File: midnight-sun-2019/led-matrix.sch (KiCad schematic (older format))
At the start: 472 parts

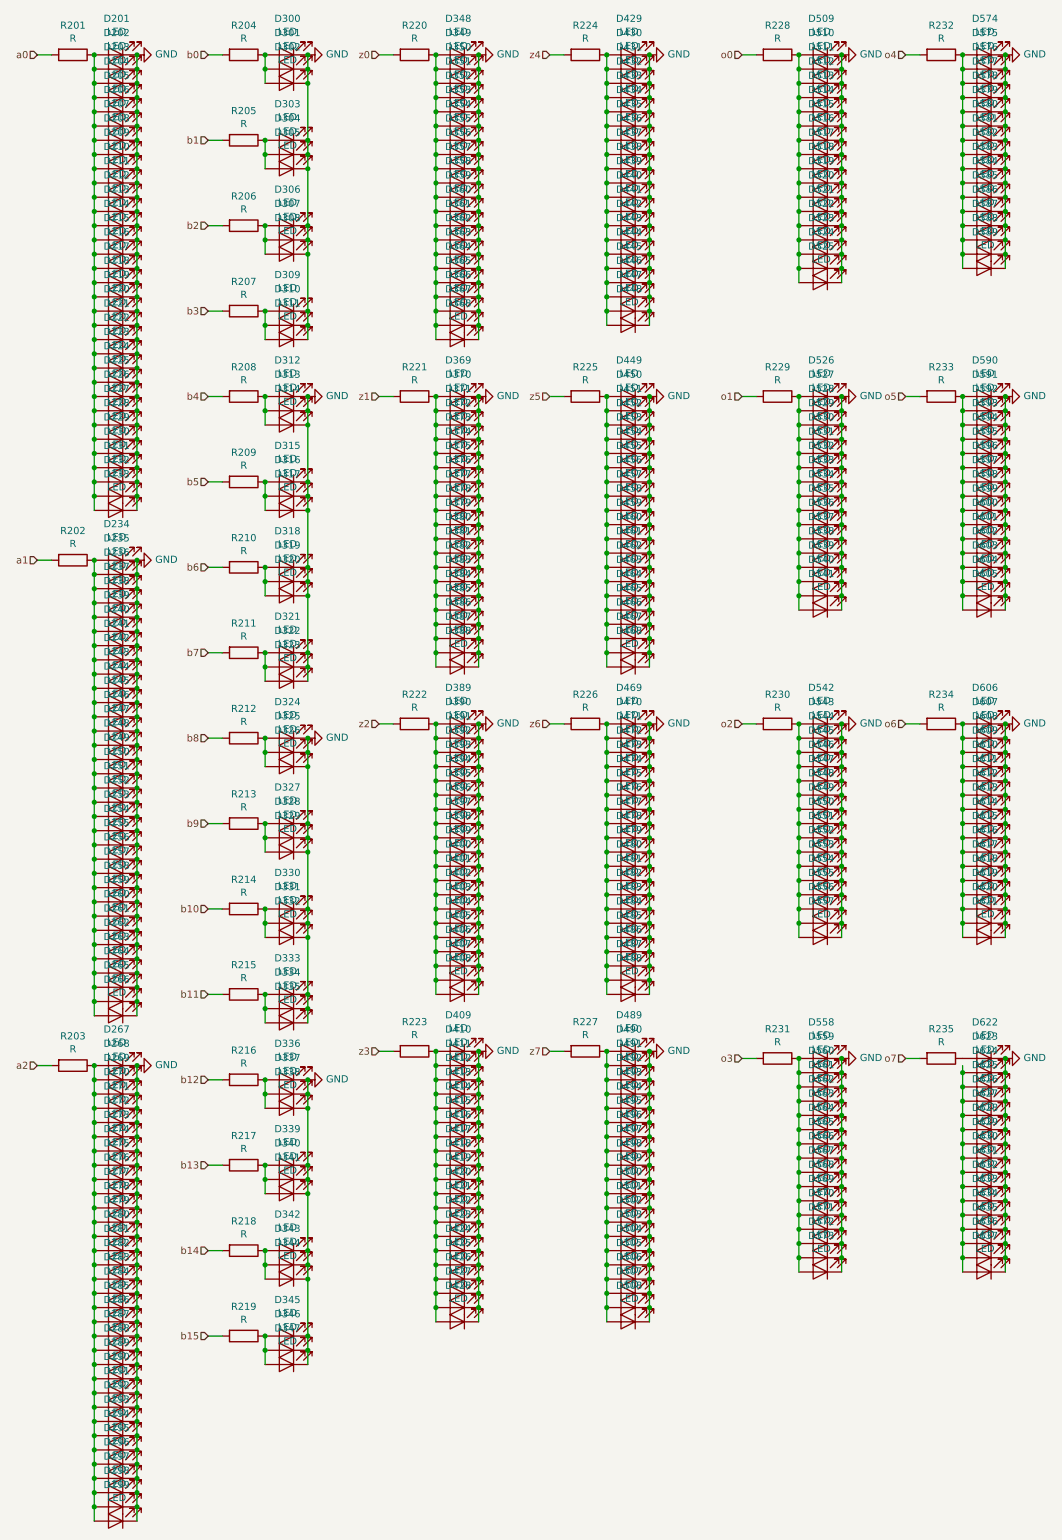
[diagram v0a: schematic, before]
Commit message: Update QR code to real flag
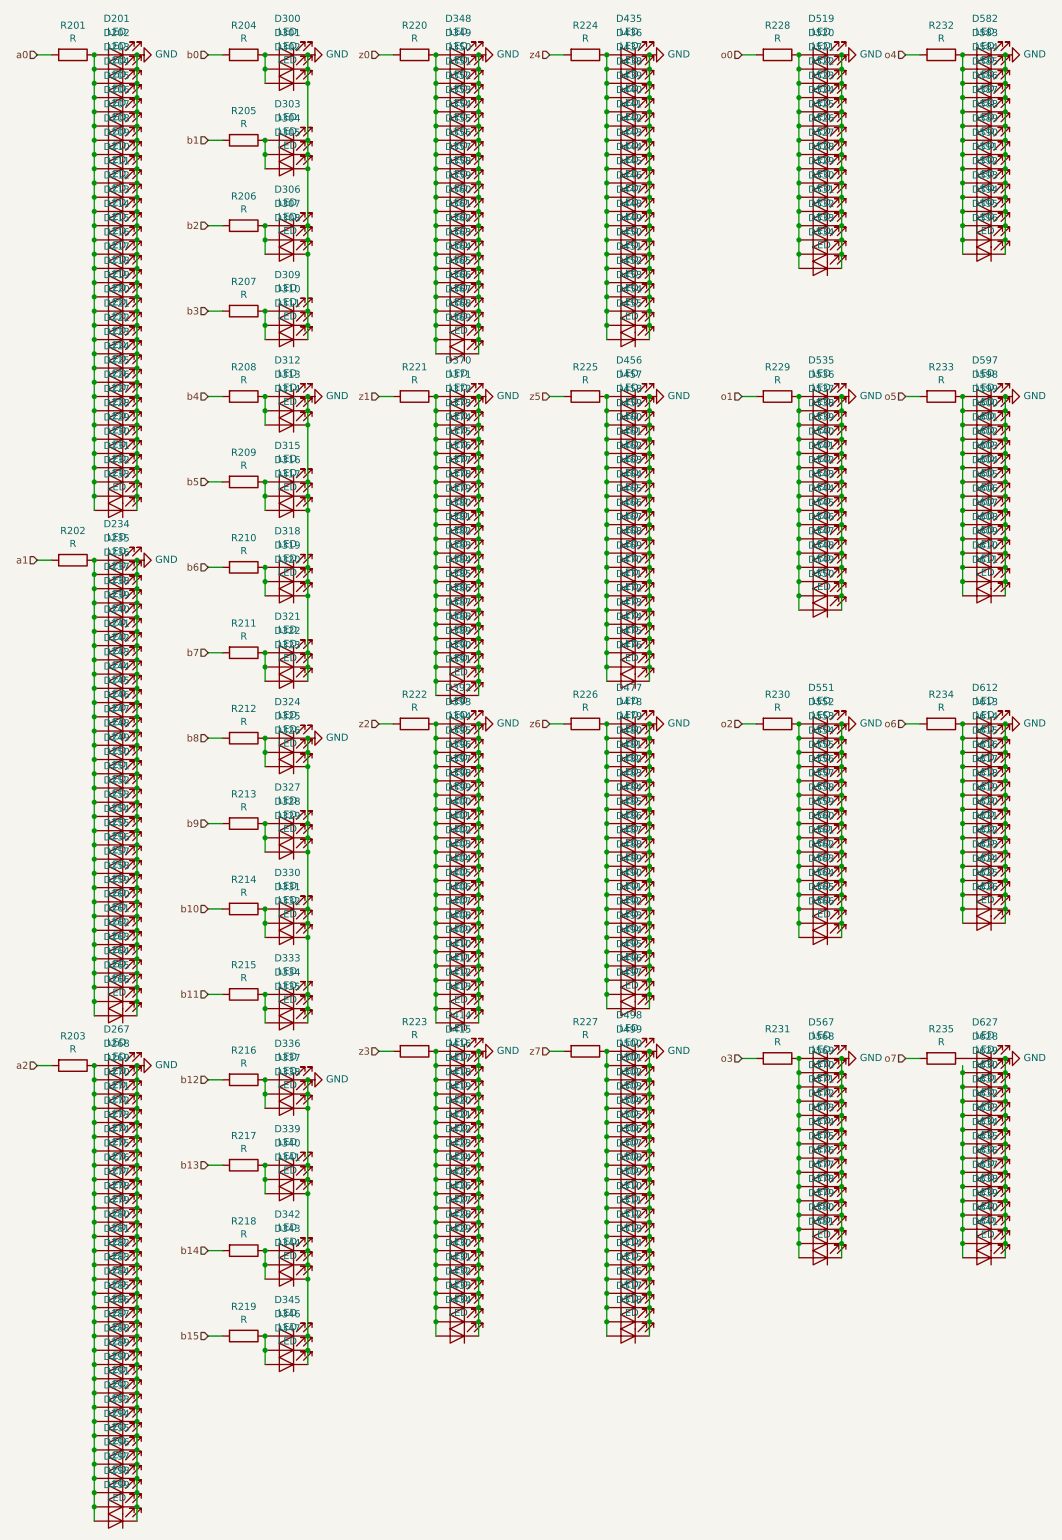
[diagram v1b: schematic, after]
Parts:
- removed D525, D573, D589, D605, D621, D637: LED, LED_SMD:LED_0805_2012Metric_Castellated, symbol Device:LED
- added D369, D390, D391, D412, D413, D434, D455, D476, D497, D518: LED, LED_SMD:LED_0805_2012Metric_Castellated, symbol Device:LED
- renumbered D369 to D370, D370 to D371, D371 to D372, D372 to D373, D373 to D374, D374 to D375, D375 to D376, D376 to D377, D377 to D378, D378 to D379, D379 to D380, D380 to D381, D381 to D382, D382 to D383, D383 to D384, D384 to D385, D385 to D386, D386 to D387, D387 to D388, D388 to D389, D389 to D392, D390 to D393, D391 to D394, D392 to D395, D393 to D396, D394 to D397, D395 to D398, D396 to D399, D397 to D400, D398 to D401, D399 to D402, D400 to D403, D401 to D404, D402 to D405, D403 to D406, D404 to D407, D405 to D408, D406 to D409, D407 to D410, D408 to D411, D409 to D414, D410 to D415, D411 to D416, D412 to D417, D413 to D418, D414 to D419, D415 to D420, D416 to D421, D417 to D422, D418 to D423, D419 to D424, D420 to D425, D421 to D426, D422 to D427, D423 to D428, D424 to D429, D425 to D430, D426 to D431, D427 to D432, D428 to D433, D429 to D435, D430 to D436, D431 to D437, D432 to D438, D433 to D439, D434 to D440, D435 to D441, D436 to D442, D437 to D443, D438 to D444, D439 to D445, D440 to D446, D441 to D447, D442 to D448, D443 to D449, D444 to D450, D445 to D451, D446 to D452, D447 to D453, D448 to D454, D449 to D456, D450 to D457, D451 to D458, D452 to D459, D453 to D460, D454 to D461, D455 to D462, D456 to D463, D457 to D464, D458 to D465, D459 to D466, D460 to D467, D461 to D468, D462 to D469, D463 to D470, D464 to D471, D465 to D472, D466 to D473, D467 to D474, D468 to D475, D469 to D477, D470 to D478, D471 to D479, D472 to D480, D473 to D481, D474 to D482, D475 to D483, D476 to D484, D477 to D485, D478 to D486, D479 to D487, D480 to D488, D481 to D489, D482 to D490, D483 to D491, D484 to D492, D485 to D493, D486 to D494, D487 to D495, D488 to D496, D489 to D498, D490 to D499, D491 to D500, D492 to D501, D493 to D502, D494 to D503, D495 to D504, D496 to D505, D497 to D506, D498 to D507, D499 to D508, D500 to D509, D501 to D510, D502 to D511, D503 to D512, D504 to D513, D505 to D514, D506 to D515, D507 to D516, D508 to D517, D509 to D519, D510 to D520, D511 to D521, D512 to D522, D513 to D523, D514 to D524, D515 to D525, D516 to D526, D517 to D527, D518 to D528, D519 to D529, D520 to D530, D521 to D531, D522 to D532, D523 to D533, D524 to D534, D526 to D535, D527 to D536, D528 to D537, D529 to D538, D530 to D539, D531 to D540, D532 to D541, D533 to D542, D534 to D543, D535 to D544, D536 to D545, D537 to D546, D538 to D547, D539 to D548, D540 to D549, D541 to D550, D542 to D551, D543 to D552, D544 to D553, D545 to D554, D546 to D555, D547 to D556, D548 to D557, D549 to D558, D550 to D559, D551 to D560, D552 to D561, D553 to D562, D554 to D563, D555 to D564, D556 to D565, D557 to D566, D558 to D567, D559 to D568, D560 to D569, D561 to D570, D562 to D571, D563 to D572, D564 to D573, D565 to D574, D566 to D575, D567 to D576, D568 to D577, D569 to D578, D570 to D579, D571 to D580, D572 to D581, D574 to D582, D575 to D583, D576 to D584, D577 to D585, D578 to D586, D579 to D587, D580 to D588, D581 to D589, D582 to D590, D583 to D591, D584 to D592, D585 to D593, D586 to D594, D587 to D595, D588 to D596, D590 to D597, D591 to D598, D592 to D599, D593 to D600, D594 to D601, D595 to D602, D596 to D603, D597 to D604, D598 to D605, D599 to D606, D600 to D607, D601 to D608, D602 to D609, D603 to D610, D604 to D611, D606 to D612, D607 to D613, D608 to D614, D609 to D615, D610 to D616, D611 to D617, D612 to D618, D613 to D619, D614 to D620, D615 to D621, D616 to D622, D617 to D623, D618 to D624, D619 to D625, D620 to D626, D622 to D627, D623 to D628, D624 to D629, D625 to D630, D626 to D631, D627 to D632, D628 to D633, D629 to D634, D630 to D635, D631 to D636, D632 to D637, D633 to D638, D634 to D639, D635 to D640, D636 to D641
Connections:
- net GND: now also D369.1 (K), D390.1 (K), D391.1 (K), D412.1 (K), D413.1 (K), D434.1 (K), D455.1 (K), D476.1 (K), D497.1 (K), D518.1 (K)
- net at D498.2 (A), D499.2 (A), D500.2 (A)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: now also D518.2 (A)
- net at D477.2 (A), D478.2 (A), D479.2 (A)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: now also D497.2 (A)
- net at D456.2 (A), D457.2 (A), D458.2 (A)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: now also D476.2 (A)
- net at D435.2 (A), D436.2 (A), D437.2 (A)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: now also D455.2 (A)
- net at D414.2 (A), D415.2 (A), D416.2 (A)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: now also D434.2 (A)
- net at D392.2 (A), D393.2 (A), D394.2 (A)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: now also D412.2 (A), D413.2 (A)
- net at D370.2 (A), D371.2 (A), D372.2 (A)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: now also D390.2 (A), D391.2 (A)
- net at D348.2 (A), D349.2 (A), D350.2 (A)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: now also D369.2 (A)

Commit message: Swap positions of LEDs and Rs in matrix
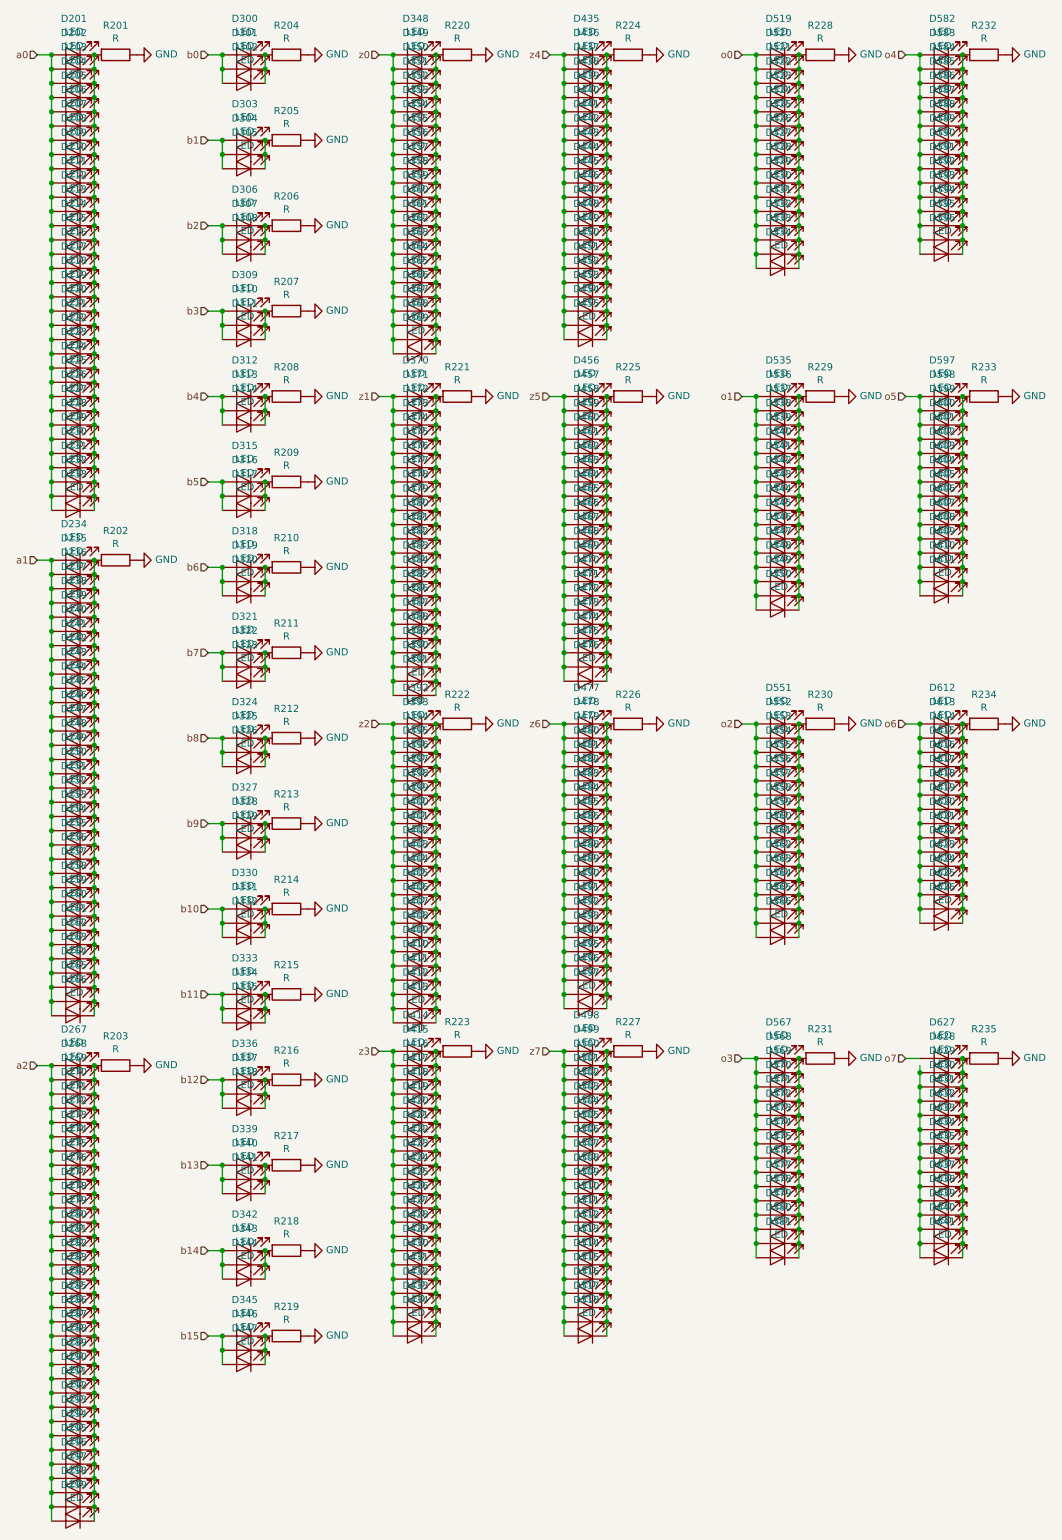
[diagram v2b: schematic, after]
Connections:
- net GND: now also R201.1, R202.1, R203.1, R204.1, R205.1, R206.1, R207.1, R208.1, R209.1, R210.1, R211.1, R212.1, R213.1, R214.1, R215.1, R216.1, R217.1, R218.1, R219.1, R220.1, R221.1, R222.1, R223.1, R224.1, R225.1, R226.1, R227.1, R228.1, R229.1, R230.1, R231.1, R232.1, R233.1, R234.1, R235.1; no longer D201.1 (K), D202.1 (K), D203.1 (K), D204.1 (K), D205.1 (K), D206.1 (K), D207.1 (K), D208.1 (K), D209.1 (K), D210.1 (K), D211.1 (K), D212.1 (K), D213.1 (K), D214.1 (K), D215.1 (K), D216.1 (K), D217.1 (K), D218.1 (K), D219.1 (K), D220.1 (K), D221.1 (K), D222.1 (K), D223.1 (K), D224.1 (K), D225.1 (K), D226.1 (K), D227.1 (K), D228.1 (K), D229.1 (K), D230.1 (K), D231.1 (K), D232.1 (K), D233.1 (K), D234.1 (K), D235.1 (K), D236.1 (K), D237.1 (K), D238.1 (K), D239.1 (K), D240.1 (K), D241.1 (K), D242.1 (K), D243.1 (K), D244.1 (K), D245.1 (K), D246.1 (K), D247.1 (K), D248.1 (K), D249.1 (K), D250.1 (K), D251.1 (K), D252.1 (K), D253.1 (K), D254.1 (K), D255.1 (K), D256.1 (K), D257.1 (K), D258.1 (K), D259.1 (K), D260.1 (K), D261.1 (K), D262.1 (K), D263.1 (K), D264.1 (K), D265.1 (K), D266.1 (K), D267.1 (K), D268.1 (K), D269.1 (K), D270.1 (K), D271.1 (K), D272.1 (K), D273.1 (K), D274.1 (K), D275.1 (K), D276.1 (K), D277.1 (K), D278.1 (K), D279.1 (K), D280.1 (K), D281.1 (K), D282.1 (K), D283.1 (K), D284.1 (K), D285.1 (K), D286.1 (K), D287.1 (K), D288.1 (K), D289.1 (K), D290.1 (K), D291.1 (K), D292.1 (K), D293.1 (K), D294.1 (K), D295.1 (K), D296.1 (K), D297.1 (K), D298.1 (K), D299.1 (K), D300.1 (K), D301.1 (K), D302.1 (K), D303.1 (K), D304.1 (K), D305.1 (K), D306.1 (K), D307.1 (K), D308.1 (K), D309.1 (K), D310.1 (K), D311.1 (K), D312.1 (K), D313.1 (K), D314.1 (K), D315.1 (K), D316.1 (K), D317.1 (K), D318.1 (K), D319.1 (K), D320.1 (K), D321.1 (K), D322.1 (K), D323.1 (K), D324.1 (K), D325.1 (K), D326.1 (K), D327.1 (K), D328.1 (K), D329.1 (K), D330.1 (K), D331.1 (K), D332.1 (K), D333.1 (K), D334.1 (K), D335.1 (K), D336.1 (K), D337.1 (K), D338.1 (K), D339.1 (K), D340.1 (K), D341.1 (K), D342.1 (K), D343.1 (K), D344.1 (K), D345.1 (K), D346.1 (K), D347.1 (K), D348.1 (K), D349.1 (K), D350.1 (K), D351.1 (K), D352.1 (K), D353.1 (K), D354.1 (K), D355.1 (K), D356.1 (K), D357.1 (K), D358.1 (K), D359.1 (K), D360.1 (K), D361.1 (K), D362.1 (K), D363.1 (K), D364.1 (K), D365.1 (K), D366.1 (K), D367.1 (K), D368.1 (K), D369.1 (K), D370.1 (K), D371.1 (K), D372.1 (K), D373.1 (K), D374.1 (K), D375.1 (K), D376.1 (K), D377.1 (K), D378.1 (K), D379.1 (K), D380.1 (K), D381.1 (K), D382.1 (K), D383.1 (K), D384.1 (K), D385.1 (K), D386.1 (K), D387.1 (K), D388.1 (K), D389.1 (K), D390.1 (K), D391.1 (K), D392.1 (K), D393.1 (K), D394.1 (K), D395.1 (K), D396.1 (K), D397.1 (K), D398.1 (K), D399.1 (K), D400.1 (K), D401.1 (K), D402.1 (K), D403.1 (K), D404.1 (K), D405.1 (K), D406.1 (K), D407.1 (K), D408.1 (K), D409.1 (K), D410.1 (K), D411.1 (K), D412.1 (K), D413.1 (K), D414.1 (K), D415.1 (K), D416.1 (K), D417.1 (K), D418.1 (K), D419.1 (K), D420.1 (K), D421.1 (K), D422.1 (K), D423.1 (K), D424.1 (K), D425.1 (K), D426.1 (K), D427.1 (K), D428.1 (K), D429.1 (K), D430.1 (K), D431.1 (K), D432.1 (K), D433.1 (K), D434.1 (K), D435.1 (K), D436.1 (K), D437.1 (K), D438.1 (K), D439.1 (K), D440.1 (K), D441.1 (K), D442.1 (K), D443.1 (K), D444.1 (K), D445.1 (K), D446.1 (K), D447.1 (K), D448.1 (K), D449.1 (K), D450.1 (K), D451.1 (K), D452.1 (K), D453.1 (K), D454.1 (K), D455.1 (K), D456.1 (K), D457.1 (K), D458.1 (K), D459.1 (K), D460.1 (K), D461.1 (K), D462.1 (K), D463.1 (K), D464.1 (K), D465.1 (K), D466.1 (K), D467.1 (K), D468.1 (K), D469.1 (K), D470.1 (K), D471.1 (K), D472.1 (K), D473.1 (K), D474.1 (K), D475.1 (K), D476.1 (K), D477.1 (K), D478.1 (K), D479.1 (K), D480.1 (K), D481.1 (K), D482.1 (K), D483.1 (K), D484.1 (K), D485.1 (K), D486.1 (K), D487.1 (K), D488.1 (K), D489.1 (K), D490.1 (K), D491.1 (K), D492.1 (K), D493.1 (K), D494.1 (K), D495.1 (K), D496.1 (K), D497.1 (K), D498.1 (K), D499.1 (K), D500.1 (K), D501.1 (K), D502.1 (K), D503.1 (K), D504.1 (K), D505.1 (K), D506.1 (K), D507.1 (K), D508.1 (K), D509.1 (K), D510.1 (K), D511.1 (K), D512.1 (K), D513.1 (K), D514.1 (K), D515.1 (K), D516.1 (K), D517.1 (K), D518.1 (K), D519.1 (K), D520.1 (K), D521.1 (K), D522.1 (K), D523.1 (K), D524.1 (K), D525.1 (K), D526.1 (K), D527.1 (K), D528.1 (K), D529.1 (K), D530.1 (K), D531.1 (K), D532.1 (K), D533.1 (K), D534.1 (K), D535.1 (K), D536.1 (K), D537.1 (K), D538.1 (K), D539.1 (K), D540.1 (K), D541.1 (K), D542.1 (K), D543.1 (K), D544.1 (K), D545.1 (K), D546.1 (K), D547.1 (K), D548.1 (K), D549.1 (K), D550.1 (K), D551.1 (K), D552.1 (K), D553.1 (K), D554.1 (K), D555.1 (K), D556.1 (K), D557.1 (K), D558.1 (K), D559.1 (K), D560.1 (K), D561.1 (K), D562.1 (K), D563.1 (K), D564.1 (K), D565.1 (K), D566.1 (K), D567.1 (K), D568.1 (K), D569.1 (K), D570.1 (K), D571.1 (K), D572.1 (K), D573.1 (K), D574.1 (K), D575.1 (K), D576.1 (K), D577.1 (K), D578.1 (K), D579.1 (K), D580.1 (K), D581.1 (K), D582.1 (K), D583.1 (K), D584.1 (K), D585.1 (K), D586.1 (K), D587.1 (K), D588.1 (K), D589.1 (K), D590.1 (K), D591.1 (K), D592.1 (K), D593.1 (K), D594.1 (K), D595.1 (K), D596.1 (K), D597.1 (K), D598.1 (K), D599.1 (K), D600.1 (K)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
- net a0: now also D201.2 (A), D202.2 (A), D203.2 (A), D204.2 (A), D205.2 (A), D206.2 (A), D207.2 (A), D208.2 (A), D209.2 (A), D210.2 (A), D211.2 (A), D212.2 (A), D213.2 (A), D214.2 (A), D215.2 (A), D216.2 (A), D217.2 (A), D218.2 (A), D219.2 (A), D220.2 (A), D221.2 (A), D222.2 (A), D223.2 (A), D224.2 (A), D225.2 (A), D226.2 (A), D227.2 (A), D228.2 (A), D229.2 (A), D230.2 (A), D231.2 (A), D232.2 (A), D233.2 (A); no longer R201.2
- net a1: now also D234.2 (A), D235.2 (A), D236.2 (A), D237.2 (A), D238.2 (A), D239.2 (A), D240.2 (A), D241.2 (A), D242.2 (A), D243.2 (A), D244.2 (A), D245.2 (A), D246.2 (A), D247.2 (A), D248.2 (A), D249.2 (A), D250.2 (A), D251.2 (A), D252.2 (A), D253.2 (A), D254.2 (A), D255.2 (A), D256.2 (A), D257.2 (A), D258.2 (A), D259.2 (A), D260.2 (A), D261.2 (A), D262.2 (A), D263.2 (A), D264.2 (A), D265.2 (A), D266.2 (A); no longer R202.2
- net a2: now also D267.2 (A), D268.2 (A), D269.2 (A), D270.2 (A), D271.2 (A), D272.2 (A), D273.2 (A), D274.2 (A), D275.2 (A), D276.2 (A), D277.2 (A), D278.2 (A), D279.2 (A), D280.2 (A), D281.2 (A), D282.2 (A), D283.2 (A), D284.2 (A), D285.2 (A), D286.2 (A), D287.2 (A), D288.2 (A), D289.2 (A), D290.2 (A), D291.2 (A), D292.2 (A), D293.2 (A), D294.2 (A), D295.2 (A), D296.2 (A), D297.2 (A), D298.2 (A), D299.2 (A); no longer R203.2
- net b0: now also D300.2 (A), D301.2 (A), D302.2 (A); no longer R204.2
- net b1: now also D303.2 (A), D304.2 (A), D305.2 (A); no longer R205.2
- net b10: now also D330.2 (A), D331.2 (A), D332.2 (A); no longer R214.2
- net b11: now also D333.2 (A), D334.2 (A), D335.2 (A); no longer R215.2
- net b12: now also D336.2 (A), D337.2 (A), D338.2 (A); no longer R216.2
- net b13: now also D339.2 (A), D340.2 (A), D341.2 (A); no longer R217.2
- net b14: now also D342.2 (A), D343.2 (A), D344.2 (A); no longer R218.2
- net b15: now also D345.2 (A), D346.2 (A), D347.2 (A); no longer R219.2
- net b2: now also D306.2 (A), D307.2 (A), D308.2 (A); no longer R206.2
- net b3: now also D309.2 (A), D310.2 (A), D311.2 (A); no longer R207.2
- net b4: now also D312.2 (A), D313.2 (A), D314.2 (A); no longer R208.2
- net b5: now also D315.2 (A), D316.2 (A), D317.2 (A); no longer R209.2
- net b6: now also D318.2 (A), D319.2 (A), D320.2 (A); no longer R210.2
- net b7: now also D321.2 (A), D322.2 (A), D323.2 (A); no longer R211.2
- net b8: now also D324.2 (A), D325.2 (A), D326.2 (A); no longer R212.2
- net b9: now also D327.2 (A), D328.2 (A), D329.2 (A); no longer R213.2
- net o0: now also D519.2 (A), D520.2 (A), D521.2 (A), D522.2 (A), D523.2 (A), D524.2 (A), D525.2 (A), D526.2 (A), D527.2 (A), D528.2 (A), D529.2 (A), D530.2 (A), D531.2 (A), D532.2 (A), D533.2 (A), D534.2 (A); no longer R228.2
- net o1: now also D535.2 (A), D536.2 (A), D537.2 (A), D538.2 (A), D539.2 (A), D540.2 (A), D541.2 (A), D542.2 (A), D543.2 (A), D544.2 (A), D545.2 (A), D546.2 (A), D547.2 (A), D548.2 (A), D549.2 (A), D550.2 (A); no longer R229.2
- net o2: now also D551.2 (A), D552.2 (A), D553.2 (A), D554.2 (A), D555.2 (A), D556.2 (A), D557.2 (A), D558.2 (A), D559.2 (A), D560.2 (A), D561.2 (A), D562.2 (A), D563.2 (A), D564.2 (A), D565.2 (A), D566.2 (A); no longer R230.2
- net o3: now also D567.2 (A), D568.2 (A), D569.2 (A), D570.2 (A), D571.2 (A), D572.2 (A), D573.2 (A), D574.2 (A), D575.2 (A), D576.2 (A), D577.2 (A), D578.2 (A), D579.2 (A), D580.2 (A), D581.2 (A); no longer R231.2
- net o4: now also D582.2 (A), D583.2 (A), D584.2 (A), D585.2 (A), D586.2 (A), D587.2 (A), D588.2 (A), D589.2 (A), D590.2 (A), D591.2 (A), D592.2 (A), D593.2 (A), D594.2 (A), D595.2 (A), D596.2 (A); no longer R232.2
- net o5: now also D597.2 (A), D598.2 (A), D599.2 (A), D600.2 (A), D601.2 (A), D602.2 (A), D603.2 (A), D604.2 (A), D605.2 (A), D606.2 (A), D607.2 (A), D608.2 (A), D609.2 (A), D610.2 (A), D611.2 (A); no longer R233.2
- net o6: now also D612.2 (A), D613.2 (A), D614.2 (A), D615.2 (A), D616.2 (A), D617.2 (A), D618.2 (A), D619.2 (A), D620.2 (A), D621.2 (A), D622.2 (A), D623.2 (A), D624.2 (A), D625.2 (A), D626.2 (A); no longer R234.2
- net o7: now also D627.2 (A); no longer R235.2
- net z0: now also D348.2 (A), D349.2 (A), D350.2 (A), D351.2 (A), D352.2 (A), D353.2 (A), D354.2 (A), D355.2 (A), D356.2 (A), D357.2 (A), D358.2 (A), D359.2 (A), D360.2 (A), D361.2 (A), D362.2 (A), D363.2 (A), D364.2 (A), D365.2 (A), D366.2 (A), D367.2 (A), D368.2 (A), D369.2 (A); no longer R220.2
- net z1: now also D370.2 (A), D371.2 (A), D372.2 (A), D373.2 (A), D374.2 (A), D375.2 (A), D376.2 (A), D377.2 (A), D378.2 (A), D379.2 (A), D380.2 (A), D381.2 (A), D382.2 (A), D383.2 (A), D384.2 (A), D385.2 (A), D386.2 (A), D387.2 (A), D388.2 (A), D389.2 (A), D390.2 (A), D391.2 (A); no longer R221.2
- net z2: now also D392.2 (A), D393.2 (A), D394.2 (A), D395.2 (A), D396.2 (A), D397.2 (A), D398.2 (A), D399.2 (A), D400.2 (A), D401.2 (A), D402.2 (A), D403.2 (A), D404.2 (A), D405.2 (A), D406.2 (A), D407.2 (A), D408.2 (A), D409.2 (A), D410.2 (A), D411.2 (A), D412.2 (A), D413.2 (A); no longer R222.2
- net z3: now also D414.2 (A), D415.2 (A), D416.2 (A), D417.2 (A), D418.2 (A), D419.2 (A), D420.2 (A), D421.2 (A), D422.2 (A), D423.2 (A), D424.2 (A), D425.2 (A), D426.2 (A), D427.2 (A), D428.2 (A), D429.2 (A), D430.2 (A), D431.2 (A), D432.2 (A), D433.2 (A), D434.2 (A); no longer R223.2
- net z4: now also D435.2 (A), D436.2 (A), D437.2 (A), D438.2 (A), D439.2 (A), D440.2 (A), D441.2 (A), D442.2 (A), D443.2 (A), D444.2 (A), D445.2 (A), D446.2 (A), D447.2 (A), D448.2 (A), D449.2 (A), D450.2 (A), D451.2 (A), D452.2 (A), D453.2 (A), D454.2 (A), D455.2 (A); no longer R224.2
- net z5: now also D456.2 (A), D457.2 (A), D458.2 (A), D459.2 (A), D460.2 (A), D461.2 (A), D462.2 (A), D463.2 (A), D464.2 (A), D465.2 (A), D466.2 (A), D467.2 (A), D468.2 (A), D469.2 (A), D470.2 (A), D471.2 (A), D472.2 (A), D473.2 (A), D474.2 (A), D475.2 (A), D476.2 (A); no longer R225.2
- net z6: now also D477.2 (A), D478.2 (A), D479.2 (A), D480.2 (A), D481.2 (A), D482.2 (A), D483.2 (A), D484.2 (A), D485.2 (A), D486.2 (A), D487.2 (A), D488.2 (A), D489.2 (A), D490.2 (A), D491.2 (A), D492.2 (A), D493.2 (A), D494.2 (A), D495.2 (A), D496.2 (A), D497.2 (A); no longer R226.2
- net z7: now also D498.2 (A), D499.2 (A), D500.2 (A), D501.2 (A), D502.2 (A), D503.2 (A), D504.2 (A), D505.2 (A), D506.2 (A), D507.2 (A), D508.2 (A), D509.2 (A), D510.2 (A), D511.2 (A), D512.2 (A), D513.2 (A), D514.2 (A), D515.2 (A), D516.2 (A), D517.2 (A), D518.2 (A); no longer R227.2
- new net: D336.1 (K), D337.1 (K), D338.1 (K), R216.2
- new net: D339.1 (K), D340.1 (K), D341.1 (K), R217.2
- new net: D342.1 (K), D343.1 (K), D344.1 (K), R218.2
- new net: D345.1 (K), D346.1 (K), D347.1 (K), R219.2
- new net: D324.1 (K), D325.1 (K), D326.1 (K), R212.2
- new net: D327.1 (K), D328.1 (K), D329.1 (K), R213.2
- new net: D330.1 (K), D331.1 (K), D332.1 (K), R214.2
- new net: D333.1 (K), D334.1 (K), D335.1 (K), R215.2
- new net: D348.1 (K), D349.1 (K), D350.1 (K), D351.1 (K), D352.1 (K), D353.1 (K), D354.1 (K), D355.1 (K), D356.1 (K), D357.1 (K), D358.1 (K), D359.1 (K), D360.1 (K), D361.1 (K), D362.1 (K), D363.1 (K), D364.1 (K), D365.1 (K), D366.1 (K), D367.1 (K), D368.1 (K), D369.1 (K), R220.2
- new net: D370.1 (K), D371.1 (K), D372.1 (K), D373.1 (K), D374.1 (K), D375.1 (K), D376.1 (K), D377.1 (K), D378.1 (K), D379.1 (K), D380.1 (K), D381.1 (K), D382.1 (K), D383.1 (K), D384.1 (K), D385.1 (K), D386.1 (K), D387.1 (K), D388.1 (K), D389.1 (K), D390.1 (K), D391.1 (K), R221.2
- new net: D392.1 (K), D393.1 (K), D394.1 (K), D395.1 (K), D396.1 (K), D397.1 (K), D398.1 (K), D399.1 (K), D400.1 (K), D401.1 (K), D402.1 (K), D403.1 (K), D404.1 (K), D405.1 (K), D406.1 (K), D407.1 (K), D408.1 (K), D409.1 (K), D410.1 (K), D411.1 (K), D412.1 (K), D413.1 (K), R222.2
- new net: D414.1 (K), D415.1 (K), D416.1 (K), D417.1 (K), D418.1 (K), D419.1 (K), D420.1 (K), D421.1 (K), D422.1 (K), D423.1 (K), D424.1 (K), D425.1 (K), D426.1 (K), D427.1 (K), D428.1 (K), D429.1 (K), D430.1 (K), D431.1 (K), D432.1 (K), D433.1 (K), D434.1 (K), R223.2
- new net: D435.1 (K), D436.1 (K), D437.1 (K), D438.1 (K), D439.1 (K), D440.1 (K), D441.1 (K), D442.1 (K), D443.1 (K), D444.1 (K), D445.1 (K), D446.1 (K), D447.1 (K), D448.1 (K), D449.1 (K), D450.1 (K), D451.1 (K), D452.1 (K), D453.1 (K), D454.1 (K), D455.1 (K), R224.2
- new net: D627.1 (K), D628.1 (K), D629.1 (K), D630.1 (K), D631.1 (K), D632.1 (K), D633.1 (K), D634.1 (K), D635.1 (K), D636.1 (K), D637.1 (K), D638.1 (K), D639.1 (K), D640.1 (K), D641.1 (K), R235.2
- new net: D612.1 (K), D613.1 (K), D614.1 (K), D615.1 (K), D616.1 (K), D617.1 (K), D618.1 (K), D619.1 (K), D620.1 (K), D621.1 (K), D622.1 (K), D623.1 (K), D624.1 (K), D625.1 (K), D626.1 (K), R234.2
- new net: D597.1 (K), D598.1 (K), D599.1 (K), D600.1 (K), D601.1 (K), D602.1 (K), D603.1 (K), D604.1 (K), D605.1 (K), D606.1 (K), D607.1 (K), D608.1 (K), D609.1 (K), D610.1 (K), D611.1 (K), R233.2
- new net: D582.1 (K), D583.1 (K), D584.1 (K), D585.1 (K), D586.1 (K), D587.1 (K), D588.1 (K), D589.1 (K), D590.1 (K), D591.1 (K), D592.1 (K), D593.1 (K), D594.1 (K), D595.1 (K), D596.1 (K), R232.2
- new net: D567.1 (K), D568.1 (K), D569.1 (K), D570.1 (K), D571.1 (K), D572.1 (K), D573.1 (K), D574.1 (K), D575.1 (K), D576.1 (K), D577.1 (K), D578.1 (K), D579.1 (K), D580.1 (K), D581.1 (K), R231.2
- new net: D551.1 (K), D552.1 (K), D553.1 (K), D554.1 (K), D555.1 (K), D556.1 (K), D557.1 (K), D558.1 (K), D559.1 (K), D560.1 (K), D561.1 (K), D562.1 (K), D563.1 (K), D564.1 (K), D565.1 (K), D566.1 (K), R230.2
- new net: D535.1 (K), D536.1 (K), D537.1 (K), D538.1 (K), D539.1 (K), D540.1 (K), D541.1 (K), D542.1 (K), D543.1 (K), D544.1 (K), D545.1 (K), D546.1 (K), D547.1 (K), D548.1 (K), D549.1 (K), D550.1 (K), R229.2
- new net: D519.1 (K), D520.1 (K), D521.1 (K), D522.1 (K), D523.1 (K), D524.1 (K), D525.1 (K), D526.1 (K), D527.1 (K), D528.1 (K), D529.1 (K), D530.1 (K), D531.1 (K), D532.1 (K), D533.1 (K), D534.1 (K), R228.2
- new net: D498.1 (K), D499.1 (K), D500.1 (K), D501.1 (K), D502.1 (K), D503.1 (K), D504.1 (K), D505.1 (K), D506.1 (K), D507.1 (K), D508.1 (K), D509.1 (K), D510.1 (K), D511.1 (K), D512.1 (K), D513.1 (K), D514.1 (K), D515.1 (K), D516.1 (K), D517.1 (K), D518.1 (K), R227.2
- new net: D477.1 (K), D478.1 (K), D479.1 (K), D480.1 (K), D481.1 (K), D482.1 (K), D483.1 (K), D484.1 (K), D485.1 (K), D486.1 (K), D487.1 (K), D488.1 (K), D489.1 (K), D490.1 (K), D491.1 (K), D492.1 (K), D493.1 (K), D494.1 (K), D495.1 (K), D496.1 (K), D497.1 (K), R226.2
- new net: D456.1 (K), D457.1 (K), D458.1 (K), D459.1 (K), D460.1 (K), D461.1 (K), D462.1 (K), D463.1 (K), D464.1 (K), D465.1 (K), D466.1 (K), D467.1 (K), D468.1 (K), D469.1 (K), D470.1 (K), D471.1 (K), D472.1 (K), D473.1 (K), D474.1 (K), D475.1 (K), D476.1 (K), R225.2
- new net: D312.1 (K), D313.1 (K), D314.1 (K), R208.2
- new net: D315.1 (K), D316.1 (K), D317.1 (K), R209.2
- new net: D318.1 (K), D319.1 (K), D320.1 (K), R210.2
- new net: D321.1 (K), D322.1 (K), D323.1 (K), R211.2
- new net: D300.1 (K), D301.1 (K), D302.1 (K), R204.2
- new net: D303.1 (K), D304.1 (K), D305.1 (K), R205.2
- new net: D306.1 (K), D307.1 (K), D308.1 (K), R206.2
- new net: D309.1 (K), D310.1 (K), D311.1 (K), R207.2
- new net: D267.1 (K), D268.1 (K), D269.1 (K), D270.1 (K), D271.1 (K), D272.1 (K), D273.1 (K), D274.1 (K), D275.1 (K), D276.1 (K), D277.1 (K), D278.1 (K), D279.1 (K), D280.1 (K), D281.1 (K), D282.1 (K), D283.1 (K), D284.1 (K), D285.1 (K), D286.1 (K), D287.1 (K), D288.1 (K), D289.1 (K), D290.1 (K), D291.1 (K), D292.1 (K), D293.1 (K), D294.1 (K), D295.1 (K), D296.1 (K), D297.1 (K), D298.1 (K), D299.1 (K), R203.2
- new net: D234.1 (K), D235.1 (K), D236.1 (K), D237.1 (K), D238.1 (K), D239.1 (K), D240.1 (K), D241.1 (K), D242.1 (K), D243.1 (K), D244.1 (K), D245.1 (K), D246.1 (K), D247.1 (K), D248.1 (K), D249.1 (K), D250.1 (K), D251.1 (K), D252.1 (K), D253.1 (K), D254.1 (K), D255.1 (K), D256.1 (K), D257.1 (K), D258.1 (K), D259.1 (K), D260.1 (K), D261.1 (K), D262.1 (K), D263.1 (K), D264.1 (K), D265.1 (K), D266.1 (K), R202.2
- new net: D201.1 (K), D202.1 (K), D203.1 (K), D204.1 (K), D205.1 (K), D206.1 (K), D207.1 (K), D208.1 (K), D209.1 (K), D210.1 (K), D211.1 (K), D212.1 (K), D213.1 (K), D214.1 (K), D215.1 (K), D216.1 (K), D217.1 (K), D218.1 (K), D219.1 (K), D220.1 (K), D221.1 (K), D222.1 (K), D223.1 (K), D224.1 (K), D225.1 (K), D226.1 (K), D227.1 (K), D228.1 (K), D229.1 (K), D230.1 (K), D231.1 (K), D232.1 (K), D233.1 (K), R201.2
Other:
- moved on the sheet: D201, D202, D203, D204, D205, D206, D207, D208, D209, D210, D211, D212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
